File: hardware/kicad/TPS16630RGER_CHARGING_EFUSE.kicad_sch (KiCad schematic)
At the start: 16 parts, among them U62 TPS16630RGER

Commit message: various updates
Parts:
- D36: footprint Diode_SMD:SMB -> Diode_SMD:D_SMB
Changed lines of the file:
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@@
 			)
 		)
-		(property "Footprint" "Diode_SMD:SMB"
+		(property "Footprint" "Diode_SMD:D_SMB"
 			(at 87.63 68.58 0)
 			(effects

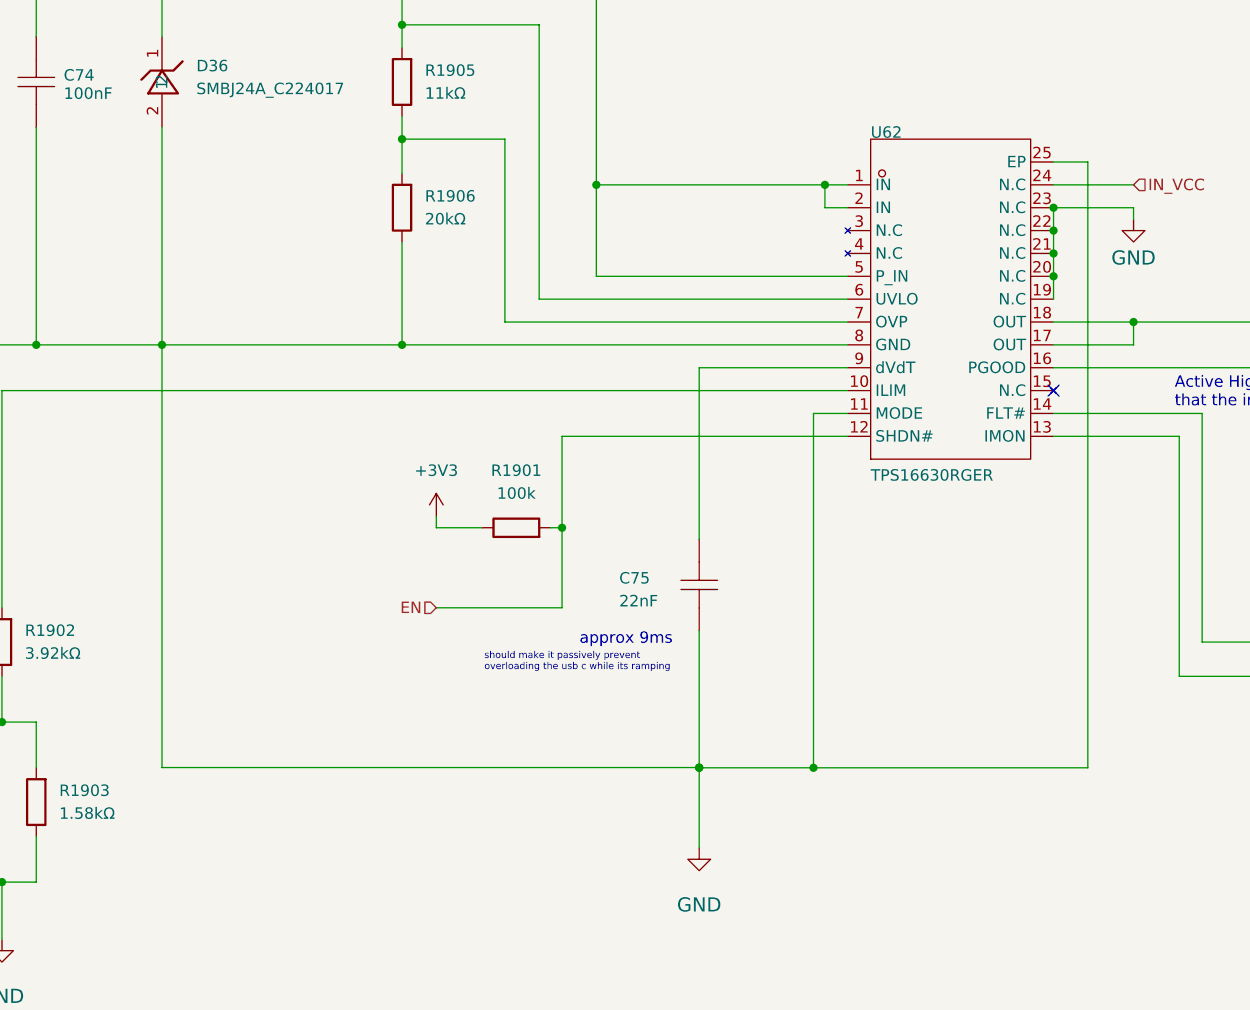
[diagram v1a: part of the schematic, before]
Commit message: update
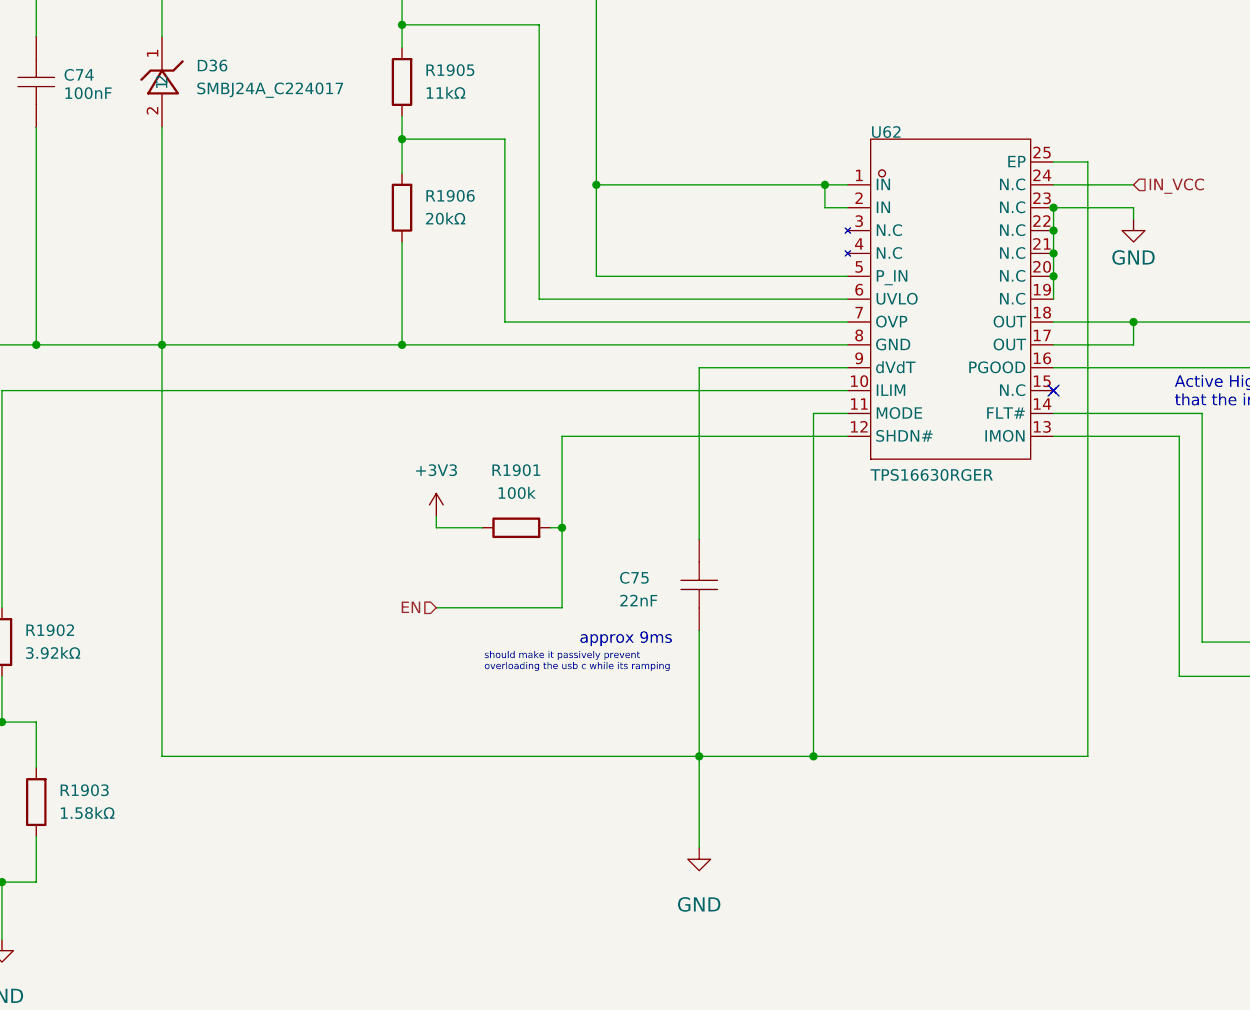
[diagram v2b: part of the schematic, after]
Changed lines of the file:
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@@
+	)
+	(junction
+		(at 160.02 143.51)
+		(diameter 0)
+		(color 0 0 0 0)
 	)
 	(junction
@@
 	)
 	(junction
-		(at 147.32 144.78)
-		(diameter 0)
-		(color 0 0 0 0)
-	)
-	(junction
 		(at 251.46 95.25)
 		(diameter 0)
@@
 	)
 	(junction
-		(at 160.02 144.78)
-		(diameter 0)
-		(color 0 0 0 0)
-	)
-	(junction
 		(at 69.85 157.48)
 		(diameter 0)
@@
 	)
 	(junction
-		(at 147.32 144.7546)
+		(at 147.32 143.51)
 		(diameter 0)
 		(color 0 0 0 0)
@@
 	(wire
 		(pts
-			(xy 160.02 144.78) (xy 147.32 144.78)
+			(xy 160.02 143.51) (xy 147.32 143.51)
 		)
 		(stroke
@@
 	(wire
 		(pts
-			(xy 147.32 153.67) (xy 147.32 144.78)
-		)
-		(stroke
-			(width 0)
-			(type default)
-		)
-	)
-	(wire
-		(pts
-			(xy 87.63 97.79) (xy 87.63 144.7546)
+			(xy 87.63 97.79) (xy 87.63 143.51)
 		)
 		(stroke
@@
 	(wire
 		(pts
-			(xy 147.32 144.78) (xy 147.32 144.7546)
-		)
-		(stroke
-			(width 0)
-			(type default)
-		)
-	)
-	(wire
-		(pts
 			(xy 125.73 74.93) (xy 114.3 74.93)
 		)
@@
 	(wire
 		(pts
+			(xy 147.32 143.51) (xy 147.32 129.54)
+		)
+		(stroke
+			(width 0)
+			(type default)
+		)
+	)
+	(wire
+		(pts
 			(xy 218.44 130.81) (xy 229.87 130.81)
 		)
@@
 	(wire
 		(pts
-			(xy 190.5 144.78) (xy 160.02 144.78)
+			(xy 190.5 143.51) (xy 160.02 143.51)
 		)
 		(stroke
@@
 	(wire
 		(pts
-			(xy 87.63 144.7546) (xy 147.32 144.7546)
-		)
-		(stroke
-			(width 0)
-			(type default)
-		)
-	)
-	(wire
-		(pts
-			(xy 147.32 144.7546) (xy 147.32 129.54)
+			(xy 87.63 143.51) (xy 147.32 143.51)
+		)
+		(stroke
+			(width 0)
+			(type default)
+		)
+	)
+	(wire
+		(pts
+			(xy 147.32 143.51) (xy 147.32 153.67)
 		)
 		(stroke
@@
 	(wire
 		(pts
-			(xy 190.5 77.47) (xy 190.5 144.78)
+			(xy 190.5 77.47) (xy 190.5 143.51)
 		)
 		(stroke
@@
 	(wire
 		(pts
-			(xy 160.02 105.41) (xy 160.02 144.78)
+			(xy 160.02 105.41) (xy 160.02 143.51)
 		)
 		(stroke
@@
 			(table_cell "MODE Pin Configuration "
 				(exclude_from_sim no)
-				(at 160.274 129.286 0)
+				(at 161.798 146.558 0)
 				(size 6.858 4.572)
 				(margins 0.9525 0.9525 0.9525 0.9525)
@@
 			(table_cell "Power Limiting, Over Current fault and Thermal Shutdown Operation"
 				(exclude_from_sim no)
-				(at 167.132 129.286 0)
+				(at 168.656 146.558 0)
 				(size 22.606 4.572)
 				(margins 0.9525 0.9525 0.9525 0.9525)
@@
 			(table_cell "Open"
 				(exclude_from_sim no)
-				(at 160.274 133.858 0)
+				(at 161.798 151.13 0)
 				(size 6.858 6.096)
 				(margins 0.9525 0.9525 0.9525 0.9525)
@@
 			(table_cell "Active Current limiting for a maximum duration of tCL_PLIM(dly). There after Latches OFF.\n\nLatch reset by toggling SHDN or UVLO low to high or power cycle"
 				(exclude_from_sim no)
-				(at 167.132 133.858 0)
+				(at 168.656 151.13 0)
 				(size 22.606 6.096)
 				(margins 0.9525 0.9525 0.9525 0.9525)
@@
 			(table_cell "Shorted to GND "
 				(exclude_from_sim no)
-				(at 160.274 139.954 0)
+				(at 161.798 157.226 0)
 				(size 6.858 3.81)
 				(margins 0.9525 0.9525 0.9525 0.9525)
@@
 			(table_cell "delay of t(TSD_retry).\nActive current limiting for a maximum duration of tCL_PLIM(dly). There after auto-retries after a"
 				(exclude_from_sim no)
-				(at 167.132 139.954 0)
+				(at 168.656 157.226 0)
 				(size 22.606 3.81)
 				(margins 0.9525 0.9525 0.9525 0.9525)

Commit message: fixes
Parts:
- U62: footprint Package_DFN_QFN:QFN-24-1EP_4x4mm_P0.5mm_EP2.8x2.8mm -> Package_DFN_QFN:Texas_RGE0024H_VQFN-24-1EP_4x4mm_P0.5mm_EP2.7x2.7mm
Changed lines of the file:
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@@
 			)
 		)
-		(property "Footprint" "Package_DFN_QFN:QFN-24-1EP_4x4mm_P0.5mm_EP2.8x2.8mm"
+		(property "Footprint" "Package_DFN_QFN:Texas_RGE0024H_VQFN-24-1EP_4x4mm_P0.5mm_EP2.7x2.7mm"
 			(at 175.26 93.98 0)
 			(effects
